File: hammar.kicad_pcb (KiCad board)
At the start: 2 copper layers, 97.5 x 53.8 mm, 115 parts, among them J1 Conn_01x08_Female, J10 YMIN, J11 ZMIN, J12 X, J13 Y, J14 Z, J15 E, J2 Conn_02x12_Odd_Even, J3 Z, J5 TEND, J7 TBED, J8 USB_C_Receptacle_USB2.0, J9 XMIN, Q1 Q_NMOS_GDS, Q2 Q_NMOS_GSD, Q3 Q_NMOS_GDS, SW1 SW_MEC_5G, SW2 SW_MEC_5G, U1 A4988, U2 ESP32-S2, U3 A4988, U4 A4988, U5 A4988, U6 3,3v lin, Y1 Crystal_GND24_Small

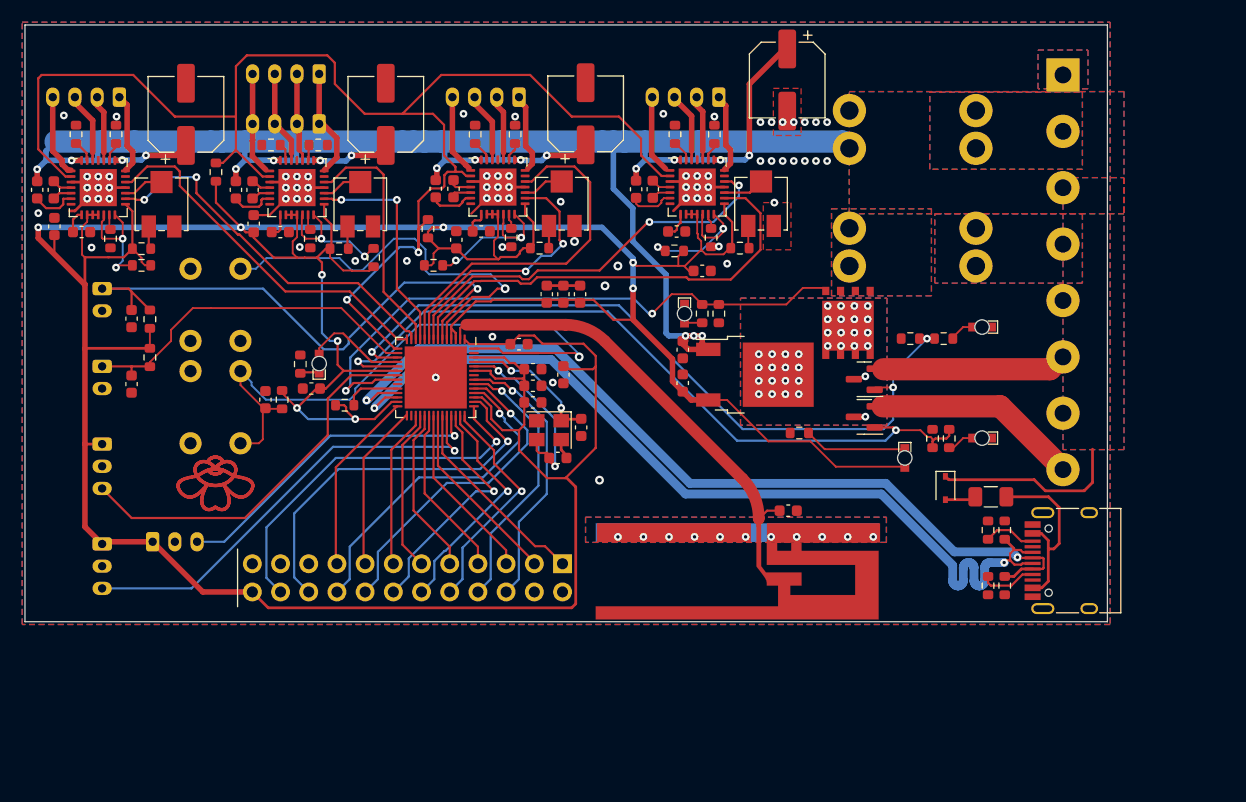
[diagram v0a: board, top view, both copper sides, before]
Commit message: Redesign
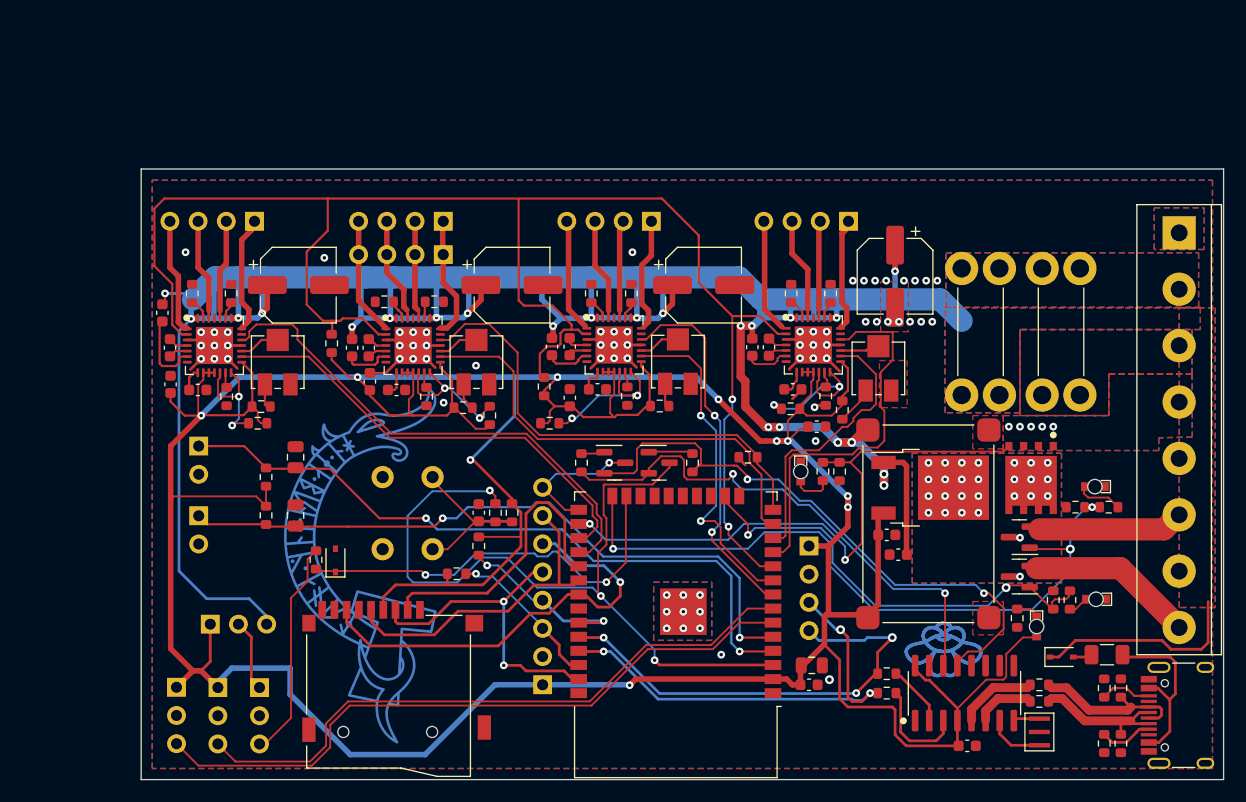
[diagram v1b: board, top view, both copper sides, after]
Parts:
- removed AE1: Antenna_Shield, MyAntennas:SWRU120B
- removed C11, C14, C5, C8, C9: 100nF, Capacitor_SMD:C_0603_1608Metric
- removed C16, C17: 1µF, Capacitor_SMD:C_0603_1608Metric
- removed C2: 15pF, Capacitor_SMD:C_0603_1608Metric
- removed C3: 1pF, Capacitor_SMD:C_0603_1608Metric
- removed SW2: SW_MEC_5G, Button_Switch_THT:SW_PUSH_6mm
- added G***: LOGO, LOGO, B.Cu at (110.8, 101.5)
- added J16: UART, Connector_PinHeader_2.54mm:PinHeader_1x04_P2.54mm_Vertical, B.Cu at (151.2, 99.7)
- added J6: Conn_01x03_Male, Connector_PinHeader_2.54mm:PinHeader_1x03_P2.54mm_Vertical, B.Cu at (97.3, 106.8)
- added Q4: Q_NPN_BEC, Package_TO_SOT_SMD:SOT-23, F.Cu at (137.7, 92.2)
- added Q5: Q_NPN_BEC, Package_TO_SOT_SMD:SOT-23, F.Cu at (133.7, 92.2)
- added R10: 22Ω, Resistor_SMD:R_0603_1608Metric, F.Cu at (172.0, 113.7)
- added R22: 1kΩ, Resistor_SMD:R_0603_1608Metric, F.Cu at (158.2, 113.0)
- added R34: 1kΩ, Resistor_SMD:R_0603_1608Metric, F.Cu at (123.0, 96.7)
- added R39: 680Ω, Resistor_SMD:R_0603_1608Metric, F.Cu at (106.8, 101.0)
- added R4: 22Ω, Resistor_SMD:R_0603_1608Metric, F.Cu at (172.0, 112.2)
- added R40: 10kΩ, Resistor_SMD:R_0603_1608Metric, F.Cu at (140.7, 92.2)
- added R41: 10kΩ, Resistor_SMD:R_0603_1608Metric, F.Cu at (130.7, 92.2)
- added R42: 10kΩ, Resistor_SMD:R_0603_1608Metric, F.Cu at (119.5, 102.2)
- added R43: 10kΩ, Resistor_SMD:R_0603_1608Metric, F.Cu at (121.5, 99.7)
- added U7: CH340G, Package_SO:SOIC-16_3.9x9.9mm_P1.27mm, F.Cu at (165.2, 113.0)
- added Z: ZMIN_probe, Connector_PinHeader_2.54mm:PinHeader_1x03_P2.54mm_Vertical, B.Cu at (101.7, 112.5)
- C1: value 15pF -> 100nF
- C15, C29, C30: footprint Capacitor_SMD:C_0603_1608Metric -> Capacitor_SMD:C_0805_2012Metric
- D5: value LED_Small -> D_Zener_~3,3v; footprint DIY:LED 0603 reverse mount -> Diode_SMD:D_SOD-323
- J11: value ZMIN -> I2C/SPI; footprint Connector_JST:JST_PH_S3B-PH-K_1x03_P2.00mm_Horizontal -> Connector_PinHeader_2.54mm:PinHeader_1x08_P2.54mm_Vertical; moved to B.Cu
- J12, J14, J15: footprint Connector_JST:JST_PH_S4B-PH-K_1x04_P2.00mm_Horizontal -> Connector_PinHeader_2.54mm:PinHeader_1x04_P2.54mm_Vertical; moved to B.Cu
- J2: value Conn_02x12_Odd_Even -> Micro_SD_Card; footprint Connector_PinHeader_2.54mm:PinHeader_2x12_P2.54mm_Vertical -> DIY:microSD
- J3: footprint Connector_JST:JST_PH_B4B-PH-K_1x04_P2.00mm_Vertical -> Connector_PinHeader_2.54mm:PinHeader_1x04_P2.54mm_Vertical; moved to B.Cu
- J5, J7: footprint Connector_JST:JST_PH_S2B-PH-K_1x02_P2.00mm_Horizontal -> Connector_PinHeader_2.54mm:PinHeader_1x02_P2.54mm_Vertical; moved to B.Cu
- Jw: renamed from J13; footprint Connector_JST:JST_PH_S4B-PH-K_1x04_P2.00mm_Horizontal -> Connector_PinHeader_2.54mm:PinHeader_1x04_P2.54mm_Vertical; moved to B.Cu
- R11: value 10kΩ -> 1kΩ
- R26: value 1kΩ -> 10kΩ
- SW1: moved to B.Cu
- U2: value ESP32-S2 -> ESP32-WROOM-32; footprint Package_DFN_QFN:QFN-56-1EP_7x7mm_P0.4mm_EP5.6x5.6mm -> RF_Module:ESP32-WROOM-32
- U6: footprint Package_TO_SOT_SMD:TO-252-2 -> DIY:mini BUCK
- X: renamed from J9; footprint Connector_JST:JST_PH_S3B-PH-K_1x03_P2.00mm_Horizontal -> Connector_PinHeader_2.54mm:PinHeader_1x03_P2.54mm_Vertical; moved to B.Cu
- Y: renamed from J10; footprint Connector_JST:JST_PH_S3B-PH-K_1x03_P2.00mm_Horizontal -> Connector_PinHeader_2.54mm:PinHeader_1x03_P2.54mm_Vertical; moved to B.Cu
- Y1: value Crystal_GND24_Small -> Resonator_Small; footprint Crystal:Crystal_SMD_3225-4Pin_3.2x2.5mm -> DIY:resonator_3,2x1,3
- moved R11 54.5 mm to (158.2, 111.2), turned to 0 degrees
- moved Y1 51.9 mm to (172.0, 116.5), turned to 90 degrees
- moved J11 45.2 mm to (127.2, 112.2), turned to 0 degrees
- moved C1 45.1 mm to (165.5, 117.7)
- moved R26 41.2 mm to (145.7, 91.7), turned to 0 degrees
- moved C15 41.1 mm to (151.5, 110.5), turned to 0 degrees
- moved C12 37.8 mm to (151.2, 112.2)
- moved U2 29.6 mm to (139.2, 104.7), turned to 180 degrees
- moved C32 26.8 mm to (159.2, 100.5), turned to 180 degrees
- moved R25 25.8 mm to (170.0, 106.2), turned to 90 degrees
- moved SW1 23.6 mm to (117.3, 100.0), turned to 90 degrees
- moved R15 23.1 mm to (124.5, 96.7)
- moved C37 22.9 mm to (158.2, 98.7), turned to 0 degrees
- moved C22 21.7 mm to (121.5, 96.7)
- moved Q2 21.6 mm to (171.2, 93.5)
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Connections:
- C1 pad 2: Net-(C1-Pad2) -> +3.3V
- C22 pad 2: RST -> Net-(C22-Pad2)
- D5 pad 1: Net-(D5-Pad1) -> Z-MIN
- D5 pad 2: IO13 -> GND
- F2 pad 2: BEDCONN-F -> VIN
- J1 pad 3: +VDC -> BEDCONN
- J1 pad 4: BEDCONN -> BEDCONN-F
- J11 pad 3: Z-MIN -> SCL
- J2 pad 1: IO33 -> unconnected-(J2-Pad1)
- J2 pad 2: IO46 -> SS
- J2 pad 3: IO32/SPID -> MOSI
- J2 pad 4: IO45 -> +3.3V
- J2 pad 5: IO31/SPIQ -> SCK
- J2 pad 6: IO44/U0RXD -> GND
- J2 pad 7: IO30/SPICLK -> MISO
- J2 pad 8: IO43/U0TXD -> unconnected-(J2-Pad8)
- J2 pad 9: IO29/SPICLK -> unconnected-(J2-Pad9)
- R11 pad 1: Net-(R11-Pad1) -> TX
- R11 pad 2: +3.3V -> Net-(R11-Pad2)
- R15 pad 2: RST -> Net-(C22-Pad2)
- R26 pad 2: Net-(D5-Pad1) -> Z-DIR
- SW1 pad 1: RST -> Net-(C22-Pad2)
- U2 pad 1: +3.3V -> GND
- U2 pad 10: Y-DIR -> E-EN
- U2 pad 11: Z-STP -> X-DIR
- U2 pad 12: Z-DIR -> X-STP
- U2 pad 13: E-STP -> Z-STP
- U2 pad 14: E-DIR -> Z-DIR
- U2 pad 15: E-EN -> GND
- U2 pad 16: T-BED -> FAN
- U2 pad 17: END -> unconnected-(U2-Pad17)
- U2 pad 18: IO13 -> unconnected-(U2-Pad18)
- U2 pad 19: FAN -> unconnected-(U2-Pad19)
- U2 pad 2: Net-(AE1-Pad1) -> +3.3V
- U2 pad 20: +3.3V -> unconnected-(U2-Pad20)
- U2 pad 21: Z-MIN -> unconnected-(U2-Pad21)
- U2 pad 22: BED -> unconnected-(U2-Pad22)
- U2 pad 23: unconnected-(U2-Pad23) -> Z-MIN
- U2 pad 24: Net-(R11-Pad1) -> END
- U2 pad 25: D- -> IO0
- U2 pad 26: D+ -> BED
- U2 pad 27: +3.3V -> E-STP
- U2 pad 28: IO21 -> E-DIR
- U2 pad 29: IO26/SPI_CS1 -> SS
- U2 pad 3: +3.3V -> RST
- U2 pad 30: unconnected-(U2-Pad30) -> SCK
- U2 pad 31: IO27/SPIHD -> MISO
- U2 pad 32: IO28/SPIWP -> unconnected-(U2-Pad32)
- U2 pad 33: IO29/SPICLK -> SDA
- U2 pad 34: IO30/SPICLK -> TX
- U2 pad 35: IO31/SPIQ -> RX
- U2 pad 36: IO32/SPID -> SCL
- U2 pad 37: IO33 -> MOSI
- U2 pad 38: X-MIN -> GND
- U2 pad 39: Y-MIN -> GND
- U2 pad 4: +3.3V -> T-END
- U2 pad 5: BOOT -> T-BED
- U2 pad 6: T-END -> X-MIN
- U2 pad 7: X-STP -> Y-MIN
- U2 pad 8: X-DIR -> Y-DIR
- Y1 pad 1: Net-(C2-Pad2) -> Net-(U7-Pad7)
- Y1 pad 3: Net-(C1-Pad2) -> Net-(U7-Pad8)
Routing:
- net +VDC: track 205.2 -> 274.1 mm, vias 19 -> 23
- net D+: track 82.5 -> 14.4 mm, vias 2 -> 0
- net D-: track 78.2 -> 13.8 mm, vias 2 -> 0
- net DTR: track 0.00 -> 54.9 mm, vias 0 -> 2
- net RTS: track 0.00 -> 47.6 mm, vias 0 -> 2
- net TX: track 0.00 -> 41.6 mm, vias 0 -> 3
- net RX: track 0.00 -> 41.1 mm, vias 0 -> 3
- net MISO: track 0.00 -> 39.1 mm, vias 0 -> 1
- net Net-(AE1-Pad1): track 38.0 -> 0.00 mm
- net BOOT: track 36.7 -> 0.00 mm, vias 1 -> 0
- net IO40/JTAG/MTDO: track 34.7 -> 0.00 mm, vias 1 -> 0
- net IO39/JTAG/MTCK: track 34.3 -> 0.00 mm, vias 1 -> 0
- net IO41/JTAG/MTDI: track 30.3 -> 0.00 mm, vias 1 -> 0
- net IO42/JTAG/MTMS: track 29.2 -> 0.00 mm, vias 1 -> 0
- net MOSI: track 0.00 -> 29.2 mm, vias 0 -> 2
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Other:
- board size 97.5 x 53.8 mm -> 97.5 x 55 mm
- board text added: "+ -"
- board text added: "- +"
- board text added: "0"
- board text added: "End"
- board text added: "Hammar v1,1"
- board text added: "MISO"
- board text added: "MOSI"
- board text added: "RX"
- board text added: "S"
- board text added: "SCK"
- board text added: "SCL"
- board text added: "SDA"
- board text added: "TX"
- board text added: "VCC"
- board text added: "VIN"
- board text added: "Z voltage 3,3V VIN"
- board text removed: "- VIN +"
- board text removed: "17"
- board text removed: "21"
- board text removed: "26"
- board text removed: "27"
- board text removed: "28"
- board text removed: "29"
- board text removed: "30"
- board text removed: "31"
- board text removed: "32"
- board text removed: "33"
- board text removed: "36"
- board text removed: "37"
- board text removed: "38"
- board text removed: "39"
- board text removed: "40"
- board text removed: "41"
- board text removed: "42"
- board text removed: "43"
- board text removed: "44"
- board text removed: "45"
- board text removed: "46"
- board text removed: "BED"
- board text removed: "END"
- board text removed: "Hammar v1"
- board text removed: "S GND 3,3V"
- board text removed: "Test"
